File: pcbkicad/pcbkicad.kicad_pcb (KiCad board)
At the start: 2 copper layers, 61 x 25.4 mm, 9 parts, among them CN1 DIP-BLACK-FEMALE-HEADER-VERT_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, CN2 DIP-BLACK-FEMALE-HEADER-VERT_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, CN3 DIP-BLACK-FEMALE-HEADER-VERT_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, J1 DIP-BLACK-FEMALE-HEADER_2X4P-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

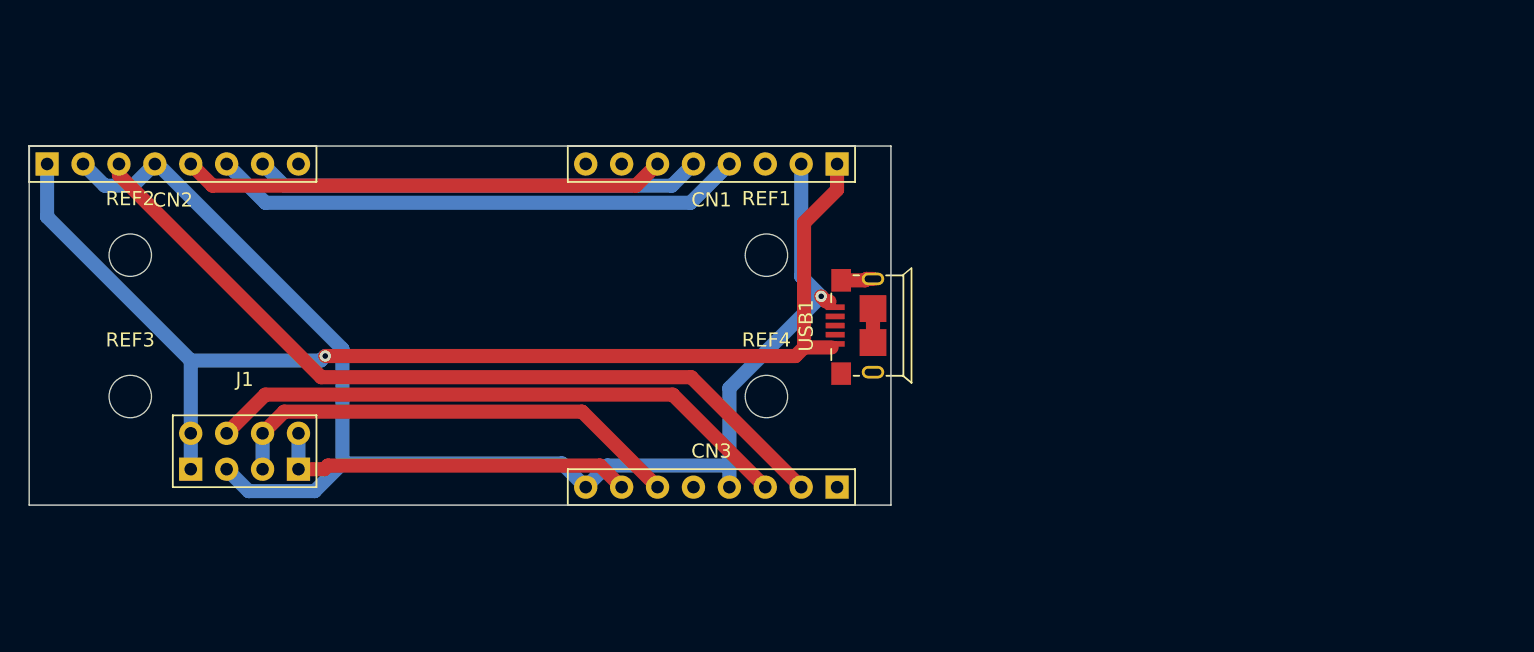
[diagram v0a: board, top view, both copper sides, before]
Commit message: update
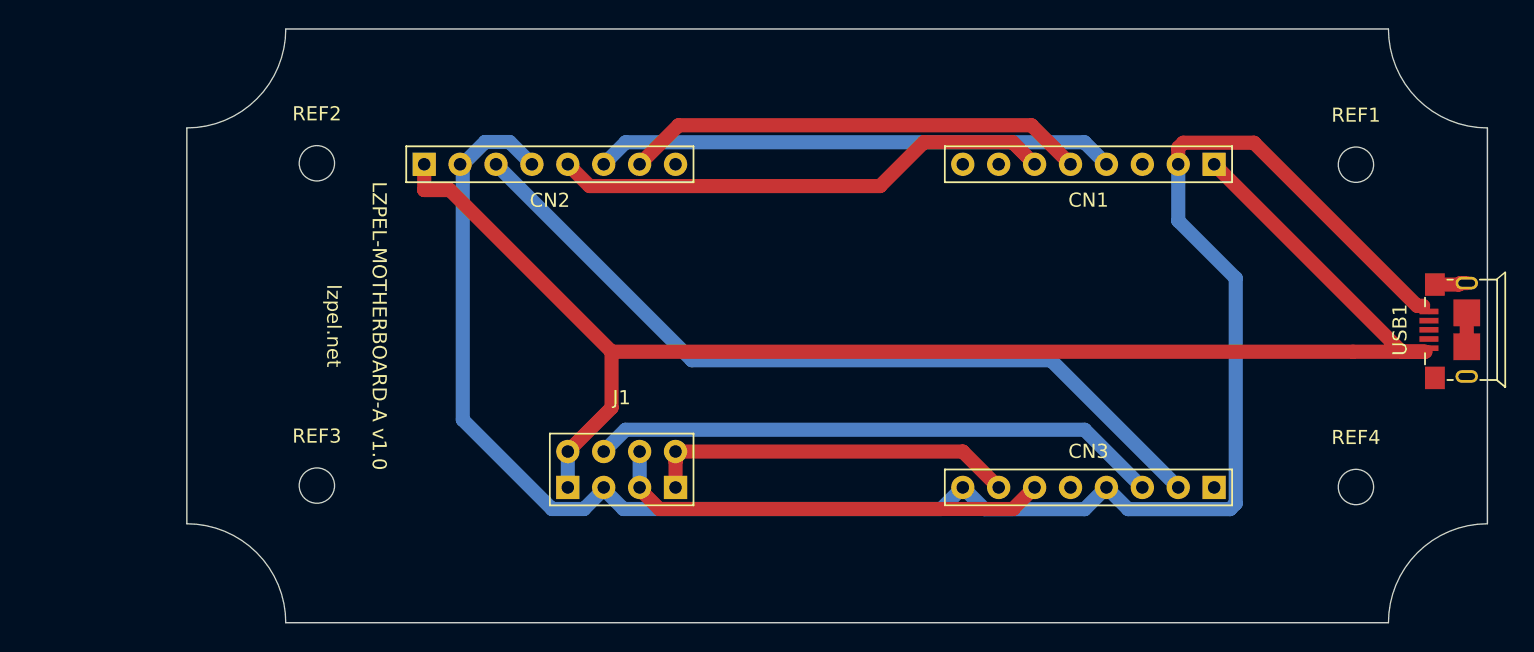
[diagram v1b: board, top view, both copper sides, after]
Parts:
- REF1, REF2, REF3, REF4: value MountingHole_3mm -> MountingHole_2.5mm; footprint MountingHole:MountingHole_3mm -> MountingHole:MountingHole_2.5mm
- moved REF1 42.2 mm to (178.9, 78.8)
- moved REF4 42.2 mm to (178.9, 101.6)
- moved USB1 42.0 mm to (186.8, 90.5)
- moved J1 26.7 mm to (127.0, 100.3)
- moved CN1 26.7 mm to (160.0, 78.8)
- moved CN2 26.7 mm to (121.9, 78.8)
- moved CN3 26.7 mm to (160.0, 101.6)
- moved REF2 14.7 mm to (105.4, 78.7)
- moved REF3 14.6 mm to (105.4, 101.5)
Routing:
- net Net-(CN1-Pad2): track 98.9 -> 135.4 mm, vias 1 -> 0
- net Net-(CN1-Pad1): track 85.8 -> 109.1 mm, vias 1 -> 0
- net Net-(CN3-Pad3): track 41.9 -> 40.4 mm
- net Net-(CN3-Pad6): track 33.3 -> 31.8 mm
- net Net-(CN1-Pad6): track 34.3 -> 35.6 mm
- net Net-(CN1-Pad5): track 31.8 -> 32.8 mm
- net Net-(CN1-Pad4): track 37.8 -> 36.9 mm
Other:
- board size 61 x 25.4 mm -> 92 x 42 mm
- rule via_min_drill: 0.3 -> 0.4
- rule via_min_size: 0.2 -> 0.4
- board text added: "LZPEL-MOTHERBOARD-A v1.0 lzpel.net"
